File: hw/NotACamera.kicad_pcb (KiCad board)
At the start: 2 copper layers, 63.4 x 52 mm, 12 parts, among them P1 SAO, U1 7555

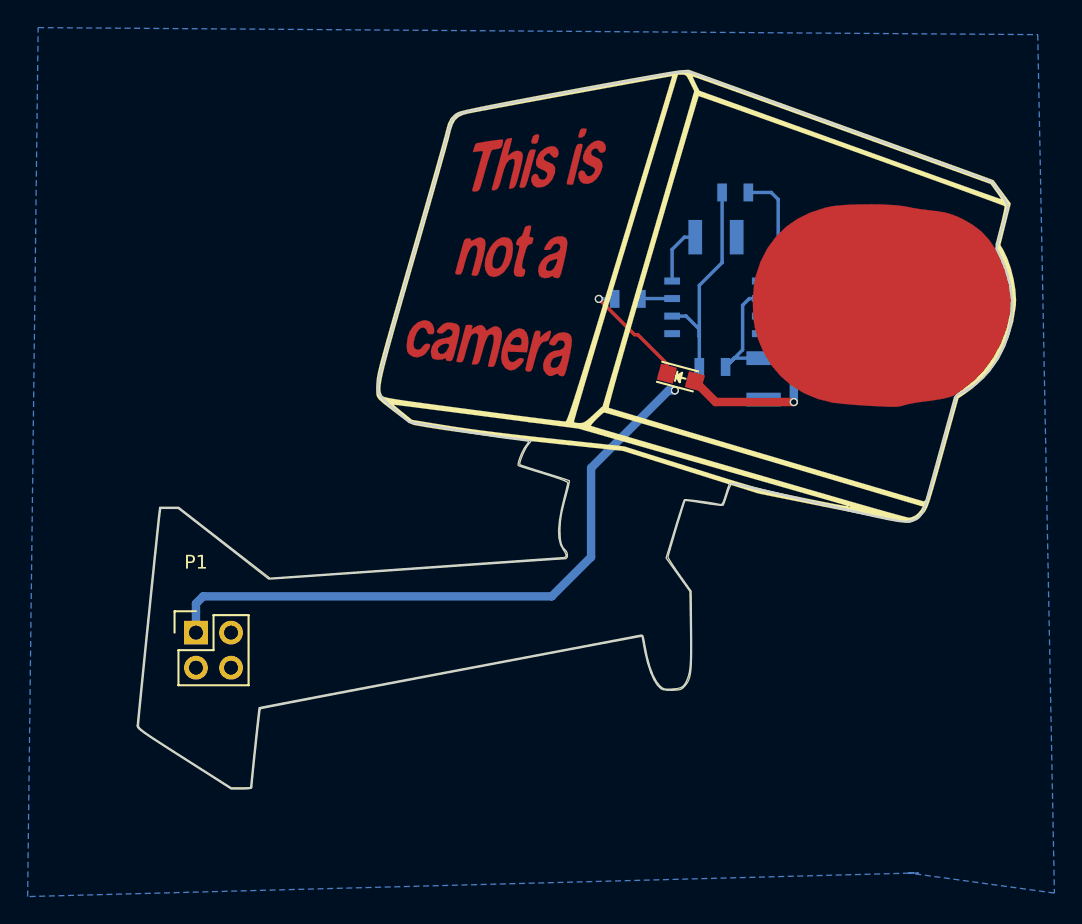
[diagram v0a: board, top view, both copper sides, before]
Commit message: Finalized version of NAC
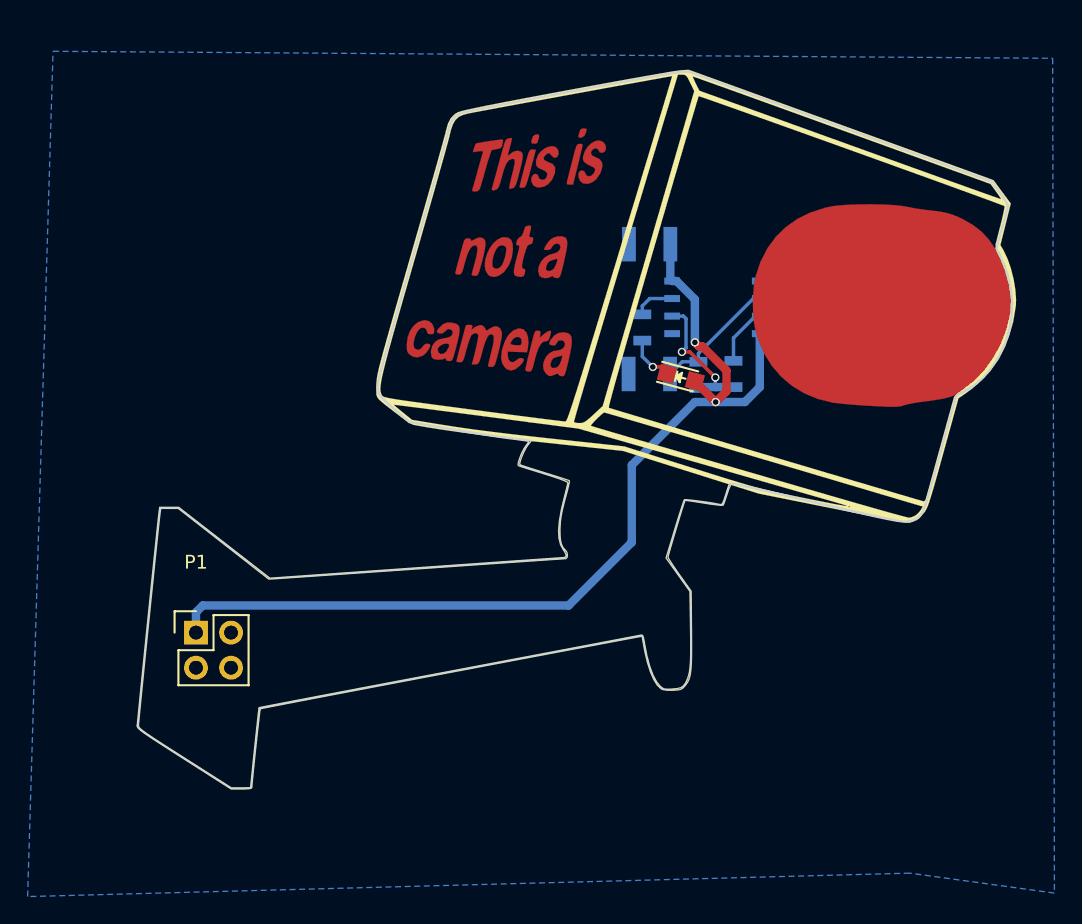
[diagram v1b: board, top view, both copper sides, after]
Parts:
- moved R2 13.1 mm to (125.7, 107.7), turned to 270 degrees
- moved C1 8.29 mm to (119.6, 107.7), turned to 180 degrees
- moved C2 4.83 mm to (119.7, 98.3), turned to 180 degrees
- moved R1 2.32 mm to (119.1, 104.3), turned to 270 degrees
- moved R3 1.17 mm to (123.2, 107.8), turned to 90 degrees
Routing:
- net Net-(R2-Pad1): track 11.9 -> 4.22 mm
- net /VCC: track 65.7 -> 72.4 mm
- net Net-(R2-Pad2): track 16.2 -> 10.1 mm, vias 0 -> 2
- net Net-(D1-Pad1): track 8.74 -> 3.45 mm
- net Net-(R1-Pad1): track 2.27 -> 2.98 mm
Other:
- board text added: "Instructions: https://contextualelectronics.com/NotACamera"
